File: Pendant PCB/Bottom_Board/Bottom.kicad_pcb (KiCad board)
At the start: 2 copper layers, 40 x 57.5 mm, 11 parts, among them J1 USB_B, J2 Conn_01x05, T1 Thumbstick_push

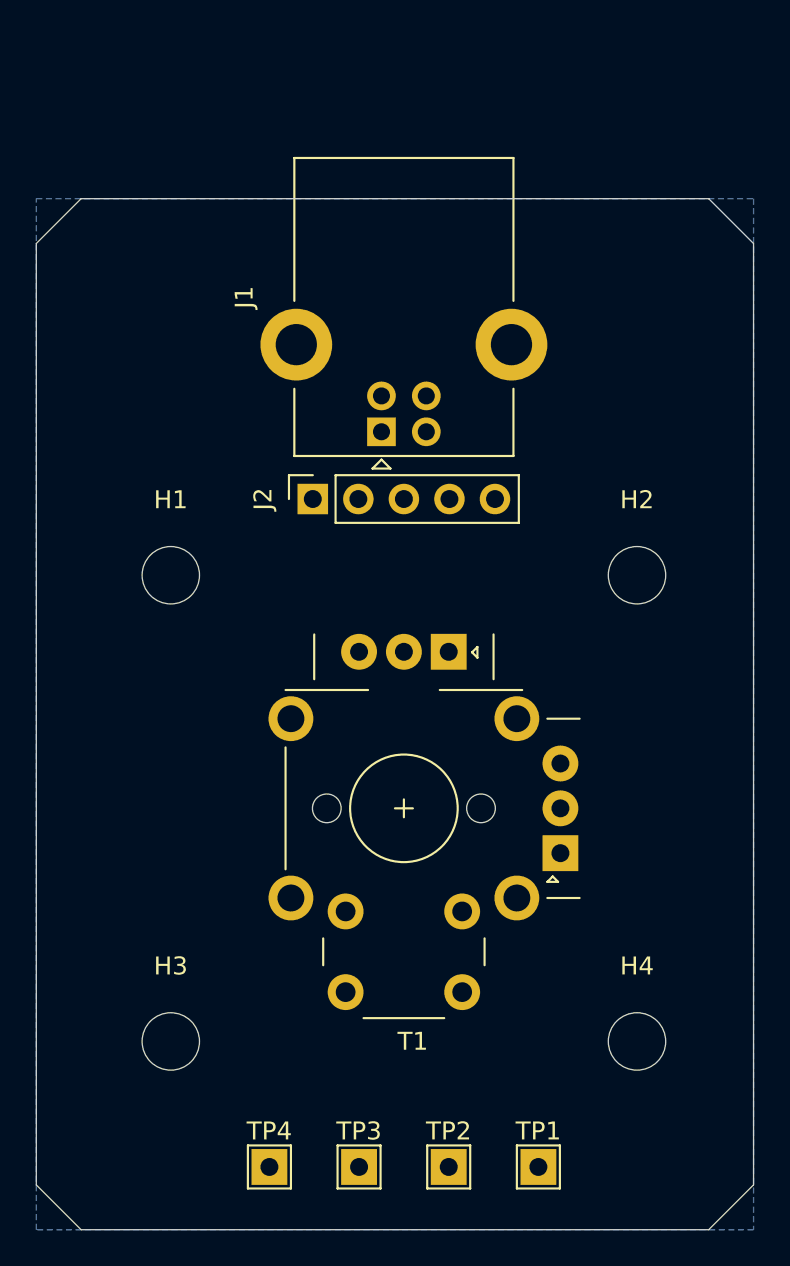
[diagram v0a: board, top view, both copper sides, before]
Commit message: Boards finished and revised. Fabrication outputs generated.
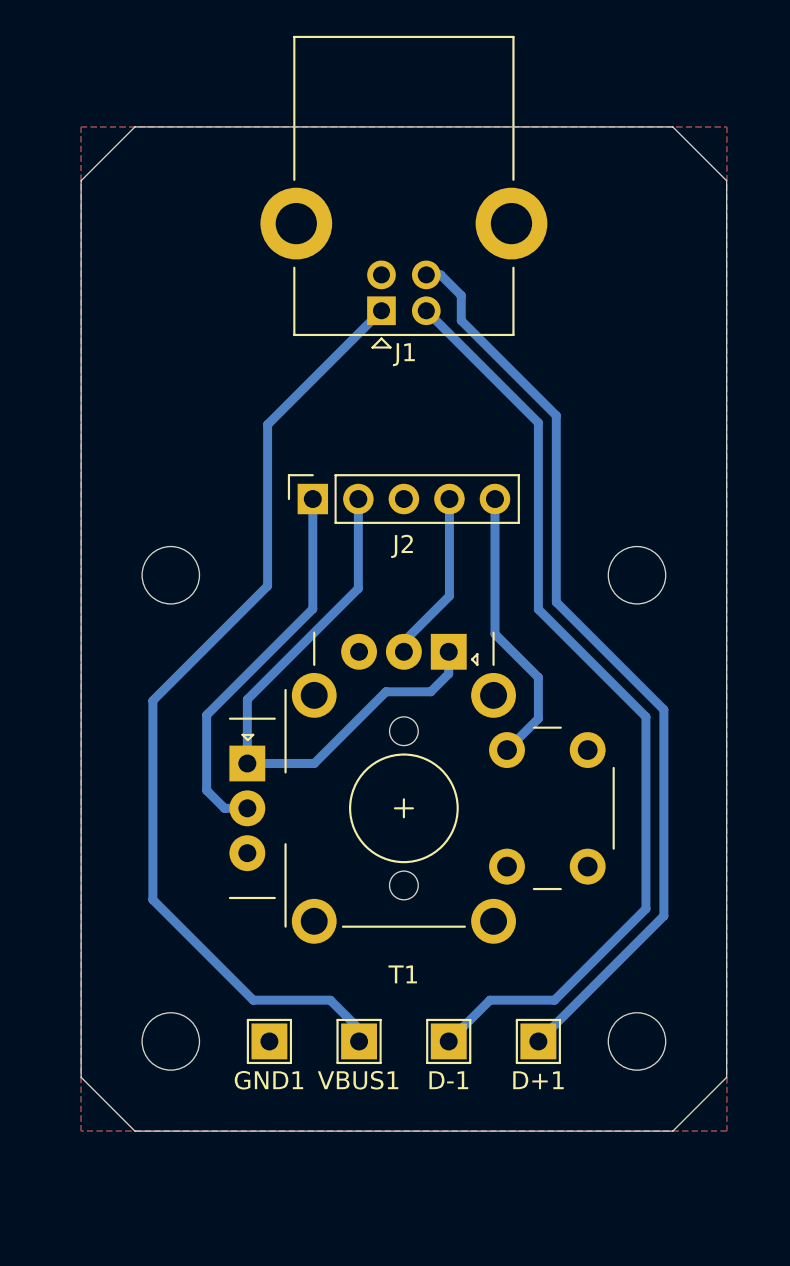
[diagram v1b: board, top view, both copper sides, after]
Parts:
- removed TP1, TP2, TP3, TP4: TestPoint, TestPoint:TestPoint_THTPad_2.0x2.0mm_Drill1.0mm
- added D+1: TestPoint, TestPoint:TestPoint_THTPad_2.0x2.0mm_Drill1.0mm, F.Cu at (107.5, 113.0)
- added D-1: TestPoint, TestPoint:TestPoint_THTPad_2.0x2.0mm_Drill1.0mm, F.Cu at (102.5, 113.0)
- added GND1: TestPoint, TestPoint:TestPoint_THTPad_2.0x2.0mm_Drill1.0mm, F.Cu at (92.5, 113.0)
- added VBUS1: TestPoint, TestPoint:TestPoint_THTPad_2.0x2.0mm_Drill1.0mm, F.Cu at (97.5, 113.0)
- moved J1 6.75 mm to (98.8, 72.2)
- turned T1 to 90 degrees
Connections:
- J1 pad 4: Net-(J1-Pad4) -> GND
- J2 pad 1: GND -> Net-(J2-Pad1)
- J2 pad 3: Net-(J2-Pad3) -> GND
- T1 pad A2: GND -> +5VA
- T1 pad B1: Net-(J2-Pad3) -> Net-(J2-Pad1)
- T1 pad C2: +5VA -> GND
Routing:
- net Net-(J1-Pad1): track 0.00 -> 53.3 mm
- net Net-(D-1-Pad1): track 0.00 -> 52.5 mm
- net Net-(D+1-Pad1): track 0.00 -> 51.6 mm
- net +5VA: track 0.00 -> 31.8 mm
- net Net-(J2-Pad1): track 0.00 -> 21.4 mm
- net Net-(J2-Pad5): track 0.00 -> 15.7 mm
- net Net-(J2-Pad4): track 0.00 -> 9.57 mm
- added copper zone on F.Cu, net GND
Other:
- board size 40 x 57.5 mm -> 36 x 56 mm
- net class Default: clearance 0.2 -> 0.47
- rule trace_clearance: 0.2 -> 0.47
